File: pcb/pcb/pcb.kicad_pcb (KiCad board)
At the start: 2 copper layers, 90 x 70 mm, 76 parts, among them J1 Conn_01x03_Pin, J10 Conn_01x03_Pin, J11 Conn_01x03_Pin, J12 Conn_01x03_Pin, J13 Conn_01x03_Pin, J14 Conn_01x03_Pin, J15 Conn_01x03_Pin, J16 Conn_01x03_Pin, J17 Conn_01x03_Pin, J18 Conn_01x04_Pin, J2 Conn_01x03_Pin, J20 Conn_01x08_Socket, J3 Conn_01x03_Pin, J4 Conn_01x03_Pin, J5 Conn_01x03_Pin, J6 Conn_01x03_Pin, J7 Conn_01x03_Pin, J8 Conn_01x03_Pin, J9 Conn_01x03_Pin, U1 Pico, U2 4052, U3 4052, U4 LM324

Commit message: cleanup pcb2
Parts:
- renumbered REF** to Hole1, REF** to Hole2, REF** to Hole3, REF** to Hole4
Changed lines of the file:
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@@
     (tags "mounting hole 3.2mm no annular m3")
     (attr exclude_from_pos_files exclude_from_bom)
-    (fp_text reference "REF**" (at 0 -4.2) (layer "F.SilkS") hide
+    (fp_text reference "Hole4" (at 0 -4.2) (layer "F.SilkS") hide
         (effects (font (size 1 1) (thickness 0.15)))
     )
@@
     (tags "mounting hole 3.2mm no annular m3")
     (attr exclude_from_pos_files exclude_from_bom)
-    (fp_text reference "REF**" (at 0 -4.2) (layer "F.SilkS") hide
+    (fp_text reference "Hole1" (at 0 -4.2) (layer "F.SilkS") hide
         (effects (font (size 1 1) (thickness 0.15)))
     )
@@
     (tags "mounting hole 3.2mm no annular m3")
     (attr exclude_from_pos_files exclude_from_bom)
-    (fp_text reference "REF**" (at 0 -4.2) (layer "F.SilkS") hide
+    (fp_text reference "Hole2" (at 0 -4.2) (layer "F.SilkS") hide
         (effects (font (size 1 1) (thickness 0.15)))
     )
@@
     (tags "mounting hole 3.2mm no annular m3")
     (attr exclude_from_pos_files exclude_from_bom)
-    (fp_text reference "REF**" (at 0 -4.2) (layer "F.SilkS") hide
+    (fp_text reference "Hole3" (at 0 -4.2) (layer "F.SilkS") hide
         (effects (font (size 1 1) (thickness 0.15)))
     )

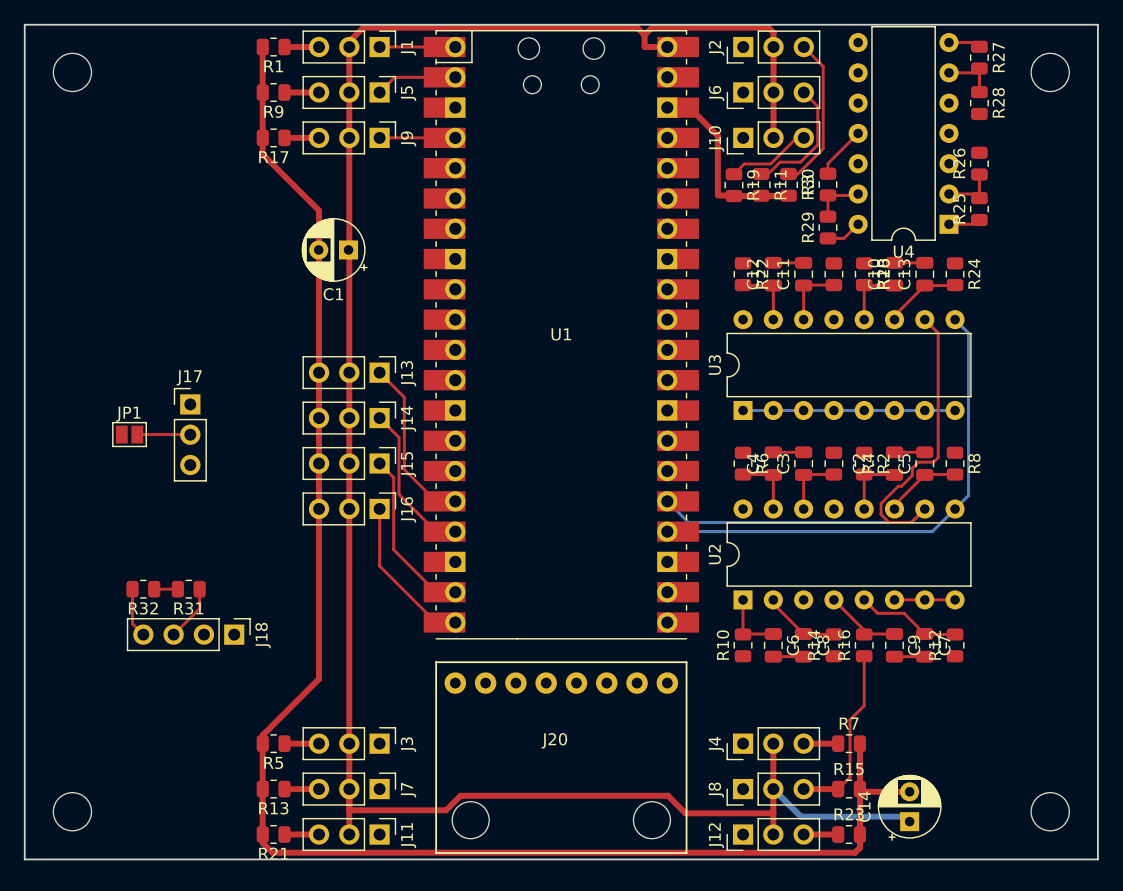
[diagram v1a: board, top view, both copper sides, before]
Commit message: autoroute
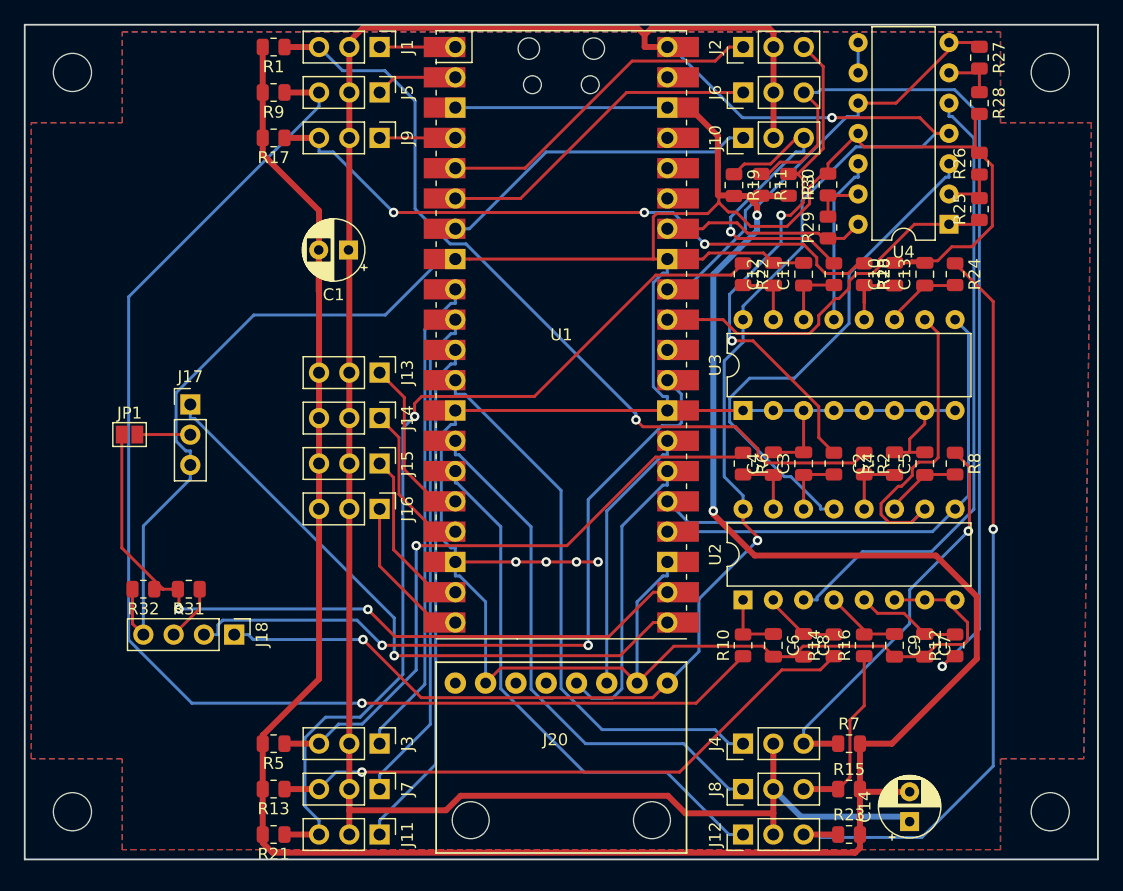
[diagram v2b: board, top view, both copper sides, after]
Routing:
- net GND: track 56.9 -> 346.0 mm, vias 0 -> 4
- net +5V: track 1.91 -> 130.1 mm, vias 0 -> 3
- net Net-(J5-Pin_3): track 2.90 -> 110.8 mm, vias 0 -> 1
- net GNDPWR: track 138.8 -> 214.1 mm, vias 0 -> 2
- net Net-(J11-Pin_3): track 2.90 -> 77.5 mm, vias 0 -> 1
- net Net-(J1-Pin_3): track 2.90 -> 69.3 mm, vias 0 -> 1
- net Net-(J6-Pin_3): track 10.6 -> 75.3 mm, vias 0 -> 1
- net Net-(J12-Pin_3): track 2.90 -> 64.9 mm, vias 0 -> 1
- net ultrason_trig: track 0.00 -> 60.8 mm, vias 0 -> 2
- net ultrason_echo: track 1.98 -> 61.7 mm, vias 0 -> 2
- net Net-(U2-Y): track 0.00 -> 52.7 mm
- net uart_tx: track 0.00 -> 52.4 mm, vias 0 -> 1
- net Net-(J9-Pin_3): track 2.90 -> 54.7 mm, vias 0 -> 3
- net Net-(J3-Pin_3): track 2.90 -> 54.7 mm, vias 0 -> 1
- net Net-(J7-Pin_3): track 2.90 -> 50.7 mm, vias 0 -> 1
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- added copper zone on B.Cu, net GND
- added copper zone on F.Cu, net GND
